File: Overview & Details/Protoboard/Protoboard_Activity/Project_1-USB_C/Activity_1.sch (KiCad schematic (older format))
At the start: 6 parts

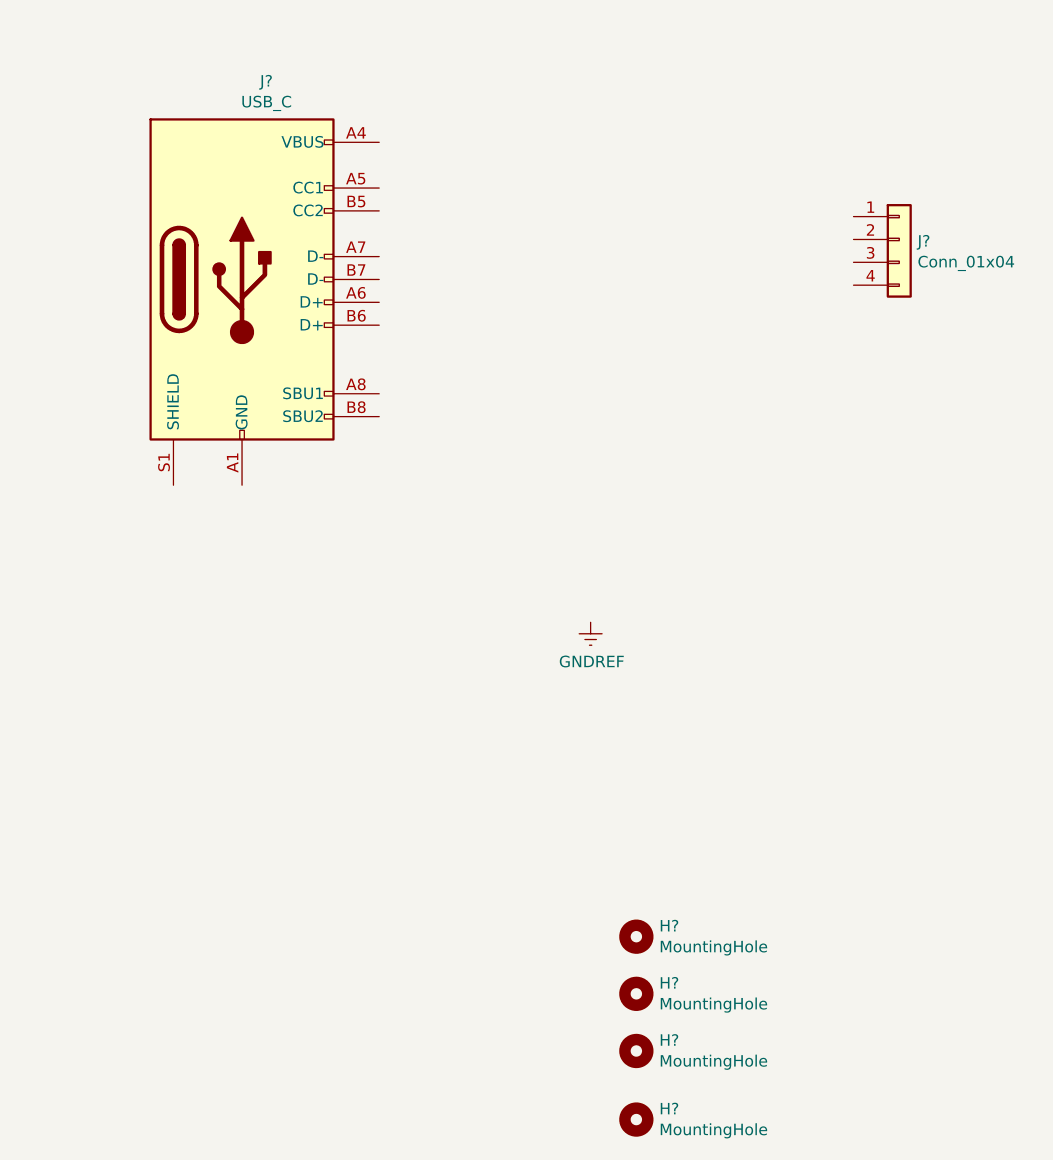
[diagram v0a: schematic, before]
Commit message: Activity 1 schematic
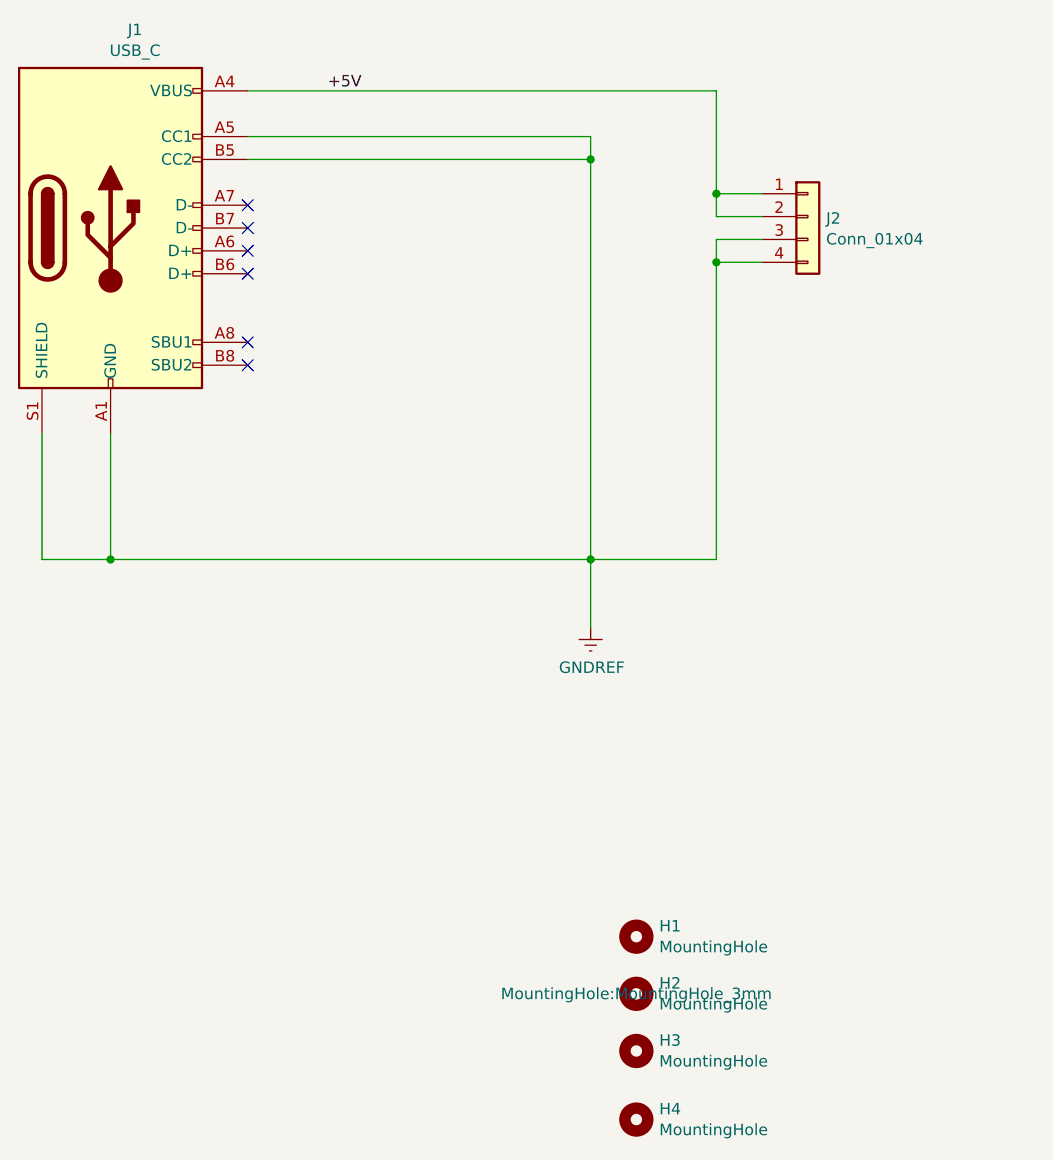
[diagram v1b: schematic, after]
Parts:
- H1, H2, H3, H4: renamed from H?; footprint (none) -> MountingHole:MountingHole_3mm
- J1: renamed from J?; footprint (none) -> intro2PCBdesign_1:USB_C_Receptacle
- J2: renamed from J?; footprint (none) -> Connector_PinHeader_2.54mm:PinHeader_1x04_P2.54mm_Vertical
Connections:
- net GNDREF: now also J1.A1 (GND), J1.A12 (GND), J1.A5 (CC1), J1.B5 (CC2), J1.S1 (SHIELD), J2.3 (Pin_3), J2.4 (Pin_4)
- net +5V: now reaches J2.1 (Pin_1)
- net +5V: now also J1.A4 (VBUS), J1.A9 (VBUS), J2.2 (Pin_2)
- no-connect marks 0 -> 6
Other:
- moved on the sheet: J1, J2
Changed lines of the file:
@@
 $EndDescr
 $Comp
-L Connector_Generic:Conn_01x04 J?
+L Connector_Generic:Conn_01x04 J2
 U 1 1 5C4787FC
-P 6150 3450
-F 0 "J?" H 6230 3442 50  0000 L CNN
-F 1 "Conn_01x04" H 6230 3351 50  0000 L CNN
-F 2 "" H 6150 3450 50  0001 C CNN
-F 3 "~" H 6150 3450 50  0001 C CNN
-	1    6150 3450
+P 5750 3350
+F 0 "J2" H 5830 3342 50  0000 L CNN
+F 1 "Conn_01x04" H 5830 3251 50  0000 L CNN
+F 2 "Connector_PinHeader_2.54mm:PinHeader_1x04_P2.54mm_Vertical" H 5750 3350 50  0001 C CNN
+F 3 "~" H 5750 3350 50  0001 C CNN
+	1    5750 3350
 	1    0    0    -1
 $EndComp
 $Comp
-L power:GNDREF #PWR?
+L power:GNDREF #PWR01
 U 1 1 5C47971A
-P 4800 5125
-F 0 "#PWR?" H 4800 4875 50  0001 C CNN
-F 1 "GNDREF" H 4805 4952 50  0000 C CNN
-F 2 "" H 4800 5125 50  0001 C CNN
-F 3 "" H 4800 5125 50  0001 C CNN
-	1    4800 5125
+P 4800 5150
+F 0 "#PWR01" H 4800 4900 50  0001 C CNN
+F 1 "GNDREF" H 4805 4977 50  0000 C CNN
+F 2 "" H 4800 5150 50  0001 C CNN
+F 3 "" H 4800 5150 50  0001 C CNN
+	1    4800 5150
 	1    0    0    -1
 $EndComp
 $Comp
-L Mechanical:MountingHole H?
+L Mechanical:MountingHole H1
 U 1 1 5C47A84A
 P 5000 6500
-F 0 "H?" H 5100 6546 50  0000 L CNN
+F 0 "H1" H 5100 6546 50  0000 L CNN
 F 1 "MountingHole" H 5100 6455 50  0000 L CNN
-F 2 "" H 5000 6500 50  0001 C CNN
+F 2 "MountingHole:MountingHole_3mm" H 5000 6500 50  0001 C CNN
 F 3 "~" H 5000 6500 50  0001 C CNN
 	1    5000 6500
@@
 $EndComp
 $Comp
-L Mechanical:MountingHole H?
+L Mechanical:MountingHole H2
 U 1 1 5C47AC98
 P 5000 6750
-F 0 "H?" H 5100 6796 50  0000 L CNN
+F 0 "H2" H 5100 6796 50  0000 L CNN
 F 1 "MountingHole" H 5100 6705 50  0000 L CNN
-F 2 "" H 5000 6750 50  0001 C CNN
+F 2 "MountingHole:MountingHole_3mm" H 5000 6750 50  0000 C CNN
 F 3 "~" H 5000 6750 50  0001 C CNN
 	1    5000 6750
@@
 $EndComp
 $Comp
-L Mechanical:MountingHole H?
+L Mechanical:MountingHole H3
 U 1 1 5C47B3EC
 P 5000 7000
-F 0 "H?" H 5100 7046 50  0000 L CNN
+F 0 "H3" H 5100 7046 50  0000 L CNN
 F 1 "MountingHole" H 5100 6955 50  0000 L CNN
-F 2 "" H 5000 7000 50  0001 C CNN
+F 2 "MountingHole:MountingHole_3mm" H 5000 7000 50  0001 C CNN
 F 3 "~" H 5000 7000 50  0001 C CNN
 	1    5000 7000
@@
 $EndComp
 $Comp
-L Mechanical:MountingHole H?
+L Mechanical:MountingHole H4
 U 1 1 5C47B5E4
 P 5000 7300
-F 0 "H?" H 5100 7346 50  0000 L CNN
+F 0 "H4" H 5100 7346 50  0000 L CNN
 F 1 "MountingHole" H 5100 7255 50  0000 L CNN
-F 2 "" H 5000 7300 50  0001 C CNN
+F 2 "MountingHole:MountingHole_3mm" H 5000 7300 50  0001 C CNN
 F 3 "~" H 5000 7300 50  0001 C CNN
 	1    5000 7300
 	1    0    0    -1
 $EndComp
+NoConn ~ 3300 3600
+NoConn ~ 3300 3500
+NoConn ~ 3300 3400
+NoConn ~ 3300 3300
 $Comp
-L Activity_1:USB_C J?
+L Activity_1:USB_C J1
 U 1 1 5E86F2D0
-P 3275 3625
-F 0 "J?" H 3382 4492 50  0000 C CNN
-F 1 "USB_C" H 3382 4401 50  0000 C CNN
-F 2 "" H 3275 4425 50  0001 C CNN
-F 3 "" H 3275 4425 50  0001 C CNN
-	1    3275 3625
+P 2700 3400
+F 0 "J1" H 2807 4267 50  0000 C CNN
+F 1 "USB_C" H 2807 4176 50  0000 C CNN
+F 2 "intro2PCBdesign_1:USB_C_Receptacle" H 2700 4200 50  0001 C CNN
+F 3 "" H 2700 4200 50  0001 C CNN
+	1    2700 3400
 	1    0    0    -1
 $EndComp
+Wire Wire Line
+	3300 2800 5350 2800
+Wire Wire Line
+	5350 2800 5350 3250
+Wire Wire Line
+	5350 3250 5550 3250
+Wire Wire Line
+	5350 3250 5350 3350
+Wire Wire Line
+	5350 3350 5550 3350
+Connection ~ 5350 3250
+Wire Wire Line
+	2400 4300 2400 4850
+Wire Wire Line
+	2400 4850 2700 4850
+Wire Wire Line
+	5350 4850 5350 3550
+Wire Wire Line
+	5350 3550 5550 3550
+Wire Wire Line
+	5350 3550 5350 3450
+Wire Wire Line
+	5350 3450 5550 3450
+Connection ~ 5350 3550
+Wire Wire Line
+	3300 3000 4800 3000
+Wire Wire Line
+	4800 3000 4800 3100
+Connection ~ 4800 4850
+Wire Wire Line
+	4800 4850 5350 4850
+Wire Wire Line
+	4800 5150 4800 4850
+Wire Wire Line
+	3300 3100 4800 3100
+Connection ~ 4800 3100
+Wire Wire Line
+	4800 3100 4800 4850
+Wire Wire Line
+	2700 4300 2700 4850
+Connection ~ 2700 4850
+Wire Wire Line
+	2700 4850 4800 4850
+NoConn ~ 3300 3900
+NoConn ~ 3300 4000
+Text Label 3650 2800 0    50   ~ 0
++5V
 $EndSCHEMATC
